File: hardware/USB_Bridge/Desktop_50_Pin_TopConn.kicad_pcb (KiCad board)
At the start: 2 copper layers, 89.2 x 82.6 mm, 108 parts, among them J1 Conn_01x03_Male, J10 Conn_01x03_Male, J11 ACK_En, J2 Conn_02x25_Odd_Even, J3 BergFloppy, J5 Conn_01x03_Male, J6 SM04B-SRSS-TB(LF)(SN), J7 TERM_BCKF, J8 EPWR, J9 Conn_01x02_Male, Q1 AO3401A, Q2 AO3401A, SW1 SW_MEC_5E, U13 LVT125, U14 LVT125, U15 LVT125, U16 LVT125, U3 AMS1117-2.85, U4 LVT245, U5 LVT245, U6 LVT245, U8 74HC14, U9 LVT245

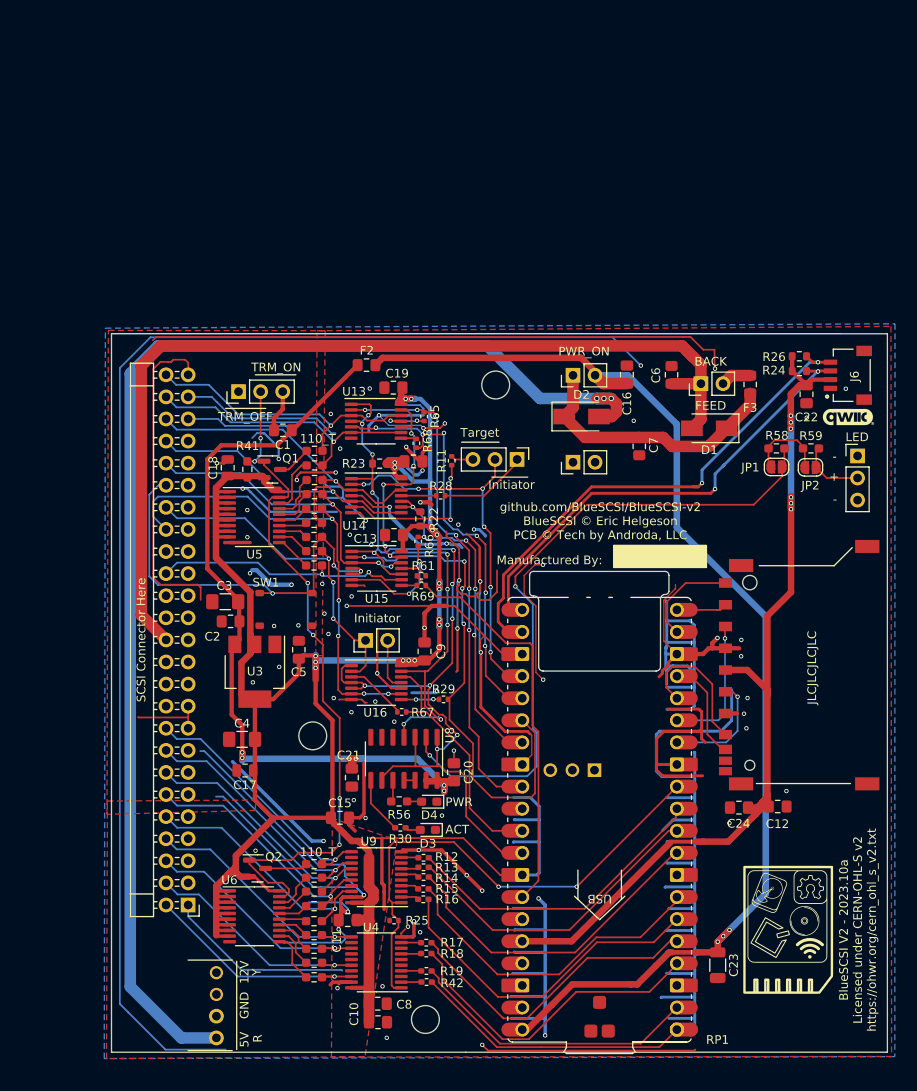
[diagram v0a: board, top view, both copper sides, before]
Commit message: intermediate checkin
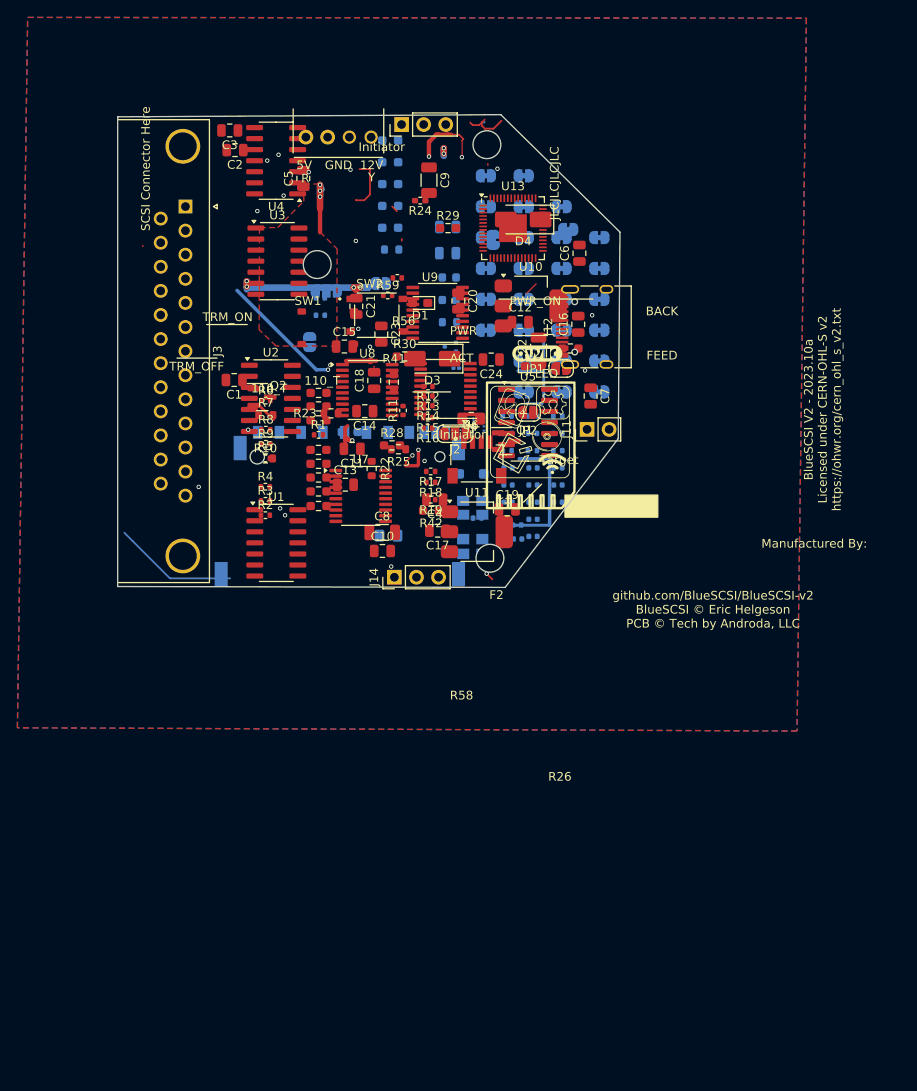
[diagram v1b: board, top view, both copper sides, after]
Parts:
- removed F3: Polyfuse, Fuse:Fuse_0805_2012Metric_Pad1.15x1.40mm_HandSolder
- removed J9: Conn_01x02_Male, Connector_PinHeader_2.54mm:PinHeader_1x02_P2.54mm_Vertical
- removed R61, R65, R66, R67, R68, R69: 1k, Resistor_SMD:R_0402_1005Metric
- removed RP1: PicoWModule, Library:Raspberry_Pi_PicoW_SMT_THT
- removed U14, U15, U16: LVT125, Package_SO:TSSOP-14_4.4x5mm_P0.65mm
- added C25: 10u 6.3V, Capacitor_SMD:C_0805_2012Metric, B.Cu at (138.6, 51.5)
- added C26: 10u 6.3V, Capacitor_SMD:C_0805_2012Metric, B.Cu at (138.6, 54.5)
- added C27: 2.2u 6.3V, Capacitor_SMD:C_0402_1005Metric, B.Cu at (151.3, 79.2)
- added C28: 100n 6.3V, Capacitor_SMD:C_0402_1005Metric, B.Cu at (151.3, 81.2)
- added C29: 100n 6.3V, Capacitor_SMD:C_0402_1005Metric, B.Cu at (151.3, 83.2)
- added C30: 100n 6.3V, Capacitor_SMD:C_0402_1005Metric, B.Cu at (144.9, 85.2)
- added C31: 2.2u 6.3V, Capacitor_SMD:C_0402_1005Metric, B.Cu at (142.1, 85.0)
- added C32: 2.2u 6.3V, Capacitor_SMD:C_0402_1005Metric, B.Cu at (146.6, 85.8)
- added C33: 100n 6.3V, Capacitor_SMD:C_0402_1005Metric, B.Cu at (148.5, 79.2)
- added C34: 100n 6.3V, Capacitor_SMD:C_0402_1005Metric, B.Cu at (148.5, 81.2)
- added C35: 100n 6.3V, Capacitor_SMD:C_0402_1005Metric, B.Cu at (148.5, 83.2)
- added C36: 100n 6.3V, Capacitor_SMD:C_0402_1005Metric, B.Cu at (148.5, 85.1)
- added C37: 100n 6.3V, Capacitor_SMD:C_0402_1005Metric, B.Cu at (148.5, 87.1)
- added C38: 2.2u 6.3V, Capacitor_SMD:C_0402_1005Metric, B.Cu at (146.7, 87.4)
- added C39: 100n 6.3V, Capacitor_SMD:C_0402_1005Metric, B.Cu at (145.6, 79.2)
- added C40: 100n 6.3V, Capacitor_SMD:C_0402_1005Metric, B.Cu at (145.6, 81.2)
- added C41: 1n 25V, Capacitor_SMD:C_0402_1005Metric, B.Cu at (145.6, 83.2)
- added D5: MBR120VLSFT1G, Diode_SMD:D_SOD-123F, B.Cu at (141.4, 79.9)
- added D6: Green, LED_SMD:LED_0603_1608Metric, B.Cu at (138.8, 57.3)
- added D7: Red, LED_SMD:LED_0603_1608Metric, B.Cu at (138.8, 59.9)
- added F1: Polyfuse, Fuse:Fuse_0805_2012Metric_Pad1.15x1.40mm_HandSolder, B.Cu at (131.8, 87.0)
- added J12: USB_C_Receptacle_USB2.0, Connector_USB:USB_C_Receptacle_HRO_TYPE-C-31-M-12, F.Cu at (155.9, 63.0)
- added J14: Debug, Connector_PinHeader_2.54mm:PinHeader_1x03_P2.54mm_Vertical, F.Cu at (132.5, 91.8)
- added J4: SM04B-SRSS-TB(LF)(SN), Library:JST_SM04B-SRSS-TB(LF)(SN), F.Cu at (142.0, 76.3)
- added JP16: SolderJumper_2_Bridged, Jumper:SolderJumper-2_P1.3mm_Bridged_RoundedPad1.0x1.5mm, B.Cu at (156.1, 52.7)
- added JP17: SolderJumper_2_Bridged, Jumper:SolderJumper-2_P1.3mm_Bridged_RoundedPad1.0x1.5mm, B.Cu at (156.1, 56.3)
- added JP18: SolderJumper_2_Bridged, Jumper:SolderJumper-2_P1.3mm_Bridged_RoundedPad1.0x1.5mm, B.Cu at (156.1, 59.8)
- added JP19: SolderJumper_2_Bridged, Jumper:SolderJumper-2_P1.3mm_Bridged_RoundedPad1.0x1.5mm, B.Cu at (156.1, 63.4)
- added JP20: SolderJumper_2_Bridged, Jumper:SolderJumper-2_P1.3mm_Bridged_RoundedPad1.0x1.5mm, B.Cu at (156.1, 66.9)
- added JP21: SolderJumper_2_Bridged, Jumper:SolderJumper-2_P1.3mm_Bridged_RoundedPad1.0x1.5mm, B.Cu at (156.1, 70.5)
- added JP24: SolderJumper_2_Bridged, Jumper:SolderJumper-2_P1.3mm_Bridged_RoundedPad1.0x1.5mm, B.Cu at (151.7, 49.2)
- added JP25: SolderJumper_2_Bridged, Jumper:SolderJumper-2_P1.3mm_Bridged_RoundedPad1.0x1.5mm, B.Cu at (151.7, 52.7)
- added JP26: SolderJumper_2_Bridged, Jumper:SolderJumper-2_P1.3mm_Bridged_RoundedPad1.0x1.5mm, B.Cu at (151.7, 56.3)
- added JP27: SolderJumper_2_Bridged, Jumper:SolderJumper-2_P1.3mm_Bridged_RoundedPad1.0x1.5mm, B.Cu at (151.7, 59.8)
- added JP28: SolderJumper_2_Bridged, Jumper:SolderJumper-2_P1.3mm_Bridged_RoundedPad1.0x1.5mm, B.Cu at (151.7, 63.4)
- added JP29: SolderJumper_2_Bridged, Jumper:SolderJumper-2_P1.3mm_Bridged_RoundedPad1.0x1.5mm, B.Cu at (151.7, 66.9)
- added JP3: SolderJumper_2_Bridged, Jumper:SolderJumper-2_P1.3mm_Bridged_RoundedPad1.0x1.5mm, B.Cu at (152.5, 51.8)
- added JP30: SolderJumper_2_Bridged, Jumper:SolderJumper-2_P1.3mm_Bridged_RoundedPad1.0x1.5mm, B.Cu at (151.7, 70.5)
- added JP32: SolderJumper_2_Bridged, Jumper:SolderJumper-2_P1.3mm_Bridged_RoundedPad1.0x1.5mm, B.Cu at (147.4, 45.6)
- added JP33: SolderJumper_2_Bridged, Jumper:SolderJumper-2_P1.3mm_Bridged_RoundedPad1.0x1.5mm, B.Cu at (147.4, 49.2)
- added JP34: SolderJumper_2_Bridged, Jumper:SolderJumper-2_P1.3mm_Bridged_RoundedPad1.0x1.5mm, B.Cu at (147.4, 52.7)
- added JP35: SolderJumper_2_Bridged, Jumper:SolderJumper-2_P1.3mm_Bridged_RoundedPad1.0x1.5mm, B.Cu at (147.4, 56.3)
- added JP36: SolderJumper_2_Bridged, Jumper:SolderJumper-2_P1.3mm_Bridged_RoundedPad1.0x1.5mm, B.Cu at (147.4, 59.8)
- added JP37: SolderJumper_2_Bridged, Jumper:SolderJumper-2_P1.3mm_Bridged_RoundedPad1.0x1.5mm, B.Cu at (147.4, 63.4)
- added JP38: SolderJumper_2_Bridged, Jumper:SolderJumper-2_P1.3mm_Bridged_RoundedPad1.0x1.5mm, B.Cu at (147.4, 66.9)
- added JP39: SolderJumper_2_Bridged, Jumper:SolderJumper-2_P1.3mm_Bridged_RoundedPad1.0x1.5mm, B.Cu at (147.4, 70.5)
- added JP40: SolderJumper_2_Bridged, Jumper:SolderJumper-2_P1.3mm_Bridged_RoundedPad1.0x1.5mm, B.Cu at (143.0, 42.1)
- added JP41: SolderJumper_2_Bridged, Jumper:SolderJumper-2_P1.3mm_Bridged_RoundedPad1.0x1.5mm, B.Cu at (143.0, 45.6)
- added JP42: SolderJumper_2_Bridged, Jumper:SolderJumper-2_P1.3mm_Bridged_RoundedPad1.0x1.5mm, B.Cu at (143.0, 49.2)
- added JP43: SolderJumper_2_Bridged, Jumper:SolderJumper-2_P1.3mm_Bridged_RoundedPad1.0x1.5mm, B.Cu at (143.0, 52.7)
- added JP44: SolderJumper_2_Bridged, Jumper:SolderJumper-2_P1.3mm_Bridged_RoundedPad1.0x1.5mm, B.Cu at (143.0, 56.3)
- added JP45: SolderJumper_2_Bridged, Jumper:SolderJumper-2_P1.3mm_Bridged_RoundedPad1.0x1.5mm, B.Cu at (143.0, 59.8)
- added JP46: SolderJumper_2_Bridged, Jumper:SolderJumper-2_P1.3mm_Bridged_RoundedPad1.0x1.5mm, B.Cu at (143.0, 63.4)
- added Q3: DMG1012T, Package_TO_SOT_SMD:SOT-523, B.Cu at (139.0, 65.3)
- added R20: 1k, Resistor_SMD:R_0402_1005Metric, B.Cu at (124.0, 59.7)
- added R21: 1k, Resistor_SMD:R_0402_1005Metric, B.Cu at (124.0, 61.7)
- added R27: 330, Resistor_SMD:R_0603_1608Metric_Pad0.98x0.95mm_HandSolder, B.Cu at (127.4, 75.1)
- added R31: 110, Resistor_SMD:R_0603_1608Metric_Pad0.98x0.95mm_HandSolder, B.Cu at (132.0, 41.6)
- added R32: 110, Resistor_SMD:R_0603_1608Metric_Pad0.98x0.95mm_HandSolder, B.Cu at (132.0, 44.1)
- added R43: 110, Resistor_SMD:R_0603_1608Metric_Pad0.98x0.95mm_HandSolder, B.Cu at (132.0, 46.6)
- added R44: 110, Resistor_SMD:R_0603_1608Metric_Pad0.98x0.95mm_HandSolder, B.Cu at (132.0, 49.1)
- added R45: 110, Resistor_SMD:R_0603_1608Metric_Pad0.98x0.95mm_HandSolder, B.Cu at (132.0, 51.6)
- added R46: 4.7k, Resistor_SMD:R_0603_1608Metric, B.Cu at (132.2, 54.1)
- added R47: 5.1k, Resistor_SMD:R_0402_1005Metric, B.Cu at (151.3, 73.3)
- added R48: 5.1k, Resistor_SMD:R_0402_1005Metric, B.Cu at (151.3, 75.3)
- added R49: 5.6k, Resistor_SMD:R_0402_1005Metric, B.Cu at (151.3, 77.2)
- added R50: 200R, Resistor_SMD:R_0603_1608Metric, B.Cu at (138.9, 62.5)
- added R51: 10k, Resistor_SMD:R_0402_1005Metric, B.Cu at (148.4, 73.3)
- added R52: 1R, Resistor_SMD:R_0402_1005Metric, B.Cu at (148.4, 75.3)
- added R53: 470R, Resistor_SMD:R_0402_1005Metric, B.Cu at (148.4, 77.2)
- added R54: 470R, Resistor_SMD:R_0402_1005Metric, B.Cu at (145.5, 73.3)
- added R55: NO-FIT, Resistor_SMD:R_0402_1005Metric, B.Cu at (145.5, 75.3)
- added R57: 27R, Resistor_SMD:R_0201_0603Metric, B.Cu at (139.6, 67.8)
- added R60: 100k, Resistor_SMD:R_0402_1005Metric, B.Cu at (145.5, 77.2)
- added SW2: TS-1187A-B-A-B, TS-1187A-B-A-B:SW_TS-1187A-B-A-B, F.Cu at (130.5, 61.7)
- added U1: LVT125, Package_SO:SO-14_3.9x8.65mm_P1.27mm, F.Cu at (119.0, 87.8)
- added U10: AMS1117-2.85, Package_TO_SOT_SMD:SOT-223-3_TabPin2, F.Cu at (148.2, 60.6)
- added U11: AMS1117-3.3, Package_TO_SOT_SMD:SOT-223-3_TabPin2, F.Cu at (142.0, 86.6)
- added U12: W25Q16JVUXIQ, agausmann:USON-8-1EP_3x2mm_P0.5mm_EP0.2x1.6mm, B.Cu at (141.6, 74.2)
- added U2: LVT125, Package_SO:SO-14_3.9x8.65mm_P1.27mm, F.Cu at (118.3, 71.2)
- added U7: LVT245, Package_SO:TSSOP-20_4.4x6.5mm_P0.65mm, F.Cu at (128.7, 82.5)
- added X1: SIT1602AI-22-33E-12.000000, Crystal:Crystal_SMD_SeikoEpson_TSX3225-4Pin_3.2x2.5mm, B.Cu at (141.5, 83.8)
- added Y1: 12MHz, Crystal:Crystal_SMD_3225-4Pin_3.2x2.5mm, B.Cu at (141.5, 88.3)
- C1, C2, C5, C7: footprint Capacitor_SMD:C_0805_2012Metric_Pad1.15x1.40mm_HandSolder -> Capacitor_SMD:C_0805_2012Metric
- C10, C15, C16: value 4.7uF -> 0.1uF; footprint Capacitor_SMD:C_0805_2012Metric_Pad1.18x1.45mm_HandSolder -> Capacitor_SMD:C_0805_2012Metric
- C11, C13, C14, C21: footprint Capacitor_SMD:C_0805_2012Metric_Pad1.18x1.45mm_HandSolder -> Capacitor_SMD:C_0805_2012Metric
- C12, C6: value 4.7uF -> 0.1uF; footprint Capacitor_SMD:C_0805_2012Metric_Pad1.15x1.40mm_HandSolder -> Capacitor_SMD:C_0805_2012Metric
- C17: value 0.1uF -> 4.7uF
- C19, C20, C24: value 0.1uF -> 4.7uF; footprint Capacitor_SMD:C_0805_2012Metric_Pad1.18x1.45mm_HandSolder -> Capacitor_SMD:C_0805_2012Metric
- C22, C8, C9: value 0.1uF -> 20uF; footprint Capacitor_SMD:C_0805_2012Metric_Pad1.18x1.45mm_HandSolder -> Capacitor_SMD:C_1206_3216Metric
- C23: value 20uF -> 0.1uF; footprint Capacitor_SMD:C_1206_3216Metric -> Capacitor_SMD:C_0805_2012Metric
- C3: value 20uF -> 4.7uF; footprint Capacitor_SMD:C_1206_3216Metric_Pad1.42x1.75mm_HandSolder -> Capacitor_SMD:C_0805_2012Metric
- C4: value 20uF -> 0.1uF; footprint Capacitor_SMD:C_1206_3216Metric_Pad1.42x1.75mm_HandSolder -> Capacitor_SMD:C_0805_2012Metric
- D1, D2: value D -> LED; footprint Diode_SMD:D_SMA -> LED_SMD:LED_0603_1608Metric_Pad1.05x0.95mm_HandSolder
- D3, D4: value LED -> D; footprint LED_SMD:LED_0603_1608Metric_Pad1.05x0.95mm_HandSolder -> Diode_SMD:D_SMA
- J1: value Conn_01x03_Male -> ACK_En; footprint Connector_PinHeader_2.54mm:PinHeader_1x03_P2.54mm_Vertical -> Jumper:SolderJumper-2_P1.3mm_Open_RoundedPad1.0x1.5mm; moved to B.Cu
- J10: value Conn_01x03_Male -> BergFloppy; footprint Connector_PinHeader_2.54mm:PinHeader_1x03_P2.54mm_Vertical -> Library:BergFloppy_RightAngle
- J11: value ACK_En -> Conn_01x02_Male
- J2: value Conn_02x25_Odd_Even -> Conn_01x03_Male; footprint Connector_PinHeader_2.54mm:PinHeader_2x25_P2.54mm_Horizontal -> Jumper:SolderJumper-3_P1.3mm_Open_RoundedPad1.0x1.5mm
- J3: value BergFloppy -> DB25_Plug_MountingHoles; footprint CustomFootprints:BergFloppy_RightAngle -> Connector_Dsub:DSUB-25_Male_Horizontal_P2.77x2.84mm_EdgePinOffset4.94mm_Housed_MountingHolesOffset7.48mm
- J6: value SM04B-SRSS-TB(LF)(SN) -> Conn_01x03_Male; footprint Library:JST_SM04B-SRSS-TB(LF)(SN) -> Jumper:SolderJumper-3_P1.3mm_Open_RoundedPad1.0x1.5mm; moved to B.Cu
- J7, J8: footprint Connector_PinHeader_2.54mm:PinHeader_1x02_P2.54mm_Vertical -> Jumper:SolderJumper-2_P1.3mm_Open_RoundedPad1.0x1.5mm; moved to B.Cu
- R1, R10, R2, R3, R4, R6, R8, R9: value 110 -> 1k; footprint Resistor_SMD:R_0603_1608Metric_Pad0.98x0.95mm_HandSolder -> Resistor_SMD:R_0402_1005Metric
- R12, R13, R14, R15, R16, R17, R18, R19: footprint Resistor_SMD:R_0402_1005Metric_Pad0.72x0.64mm_HandSolder -> Resistor_SMD:R_0402_1005Metric
- R24: value 4.7k -> 470; footprint Resistor_SMD:R_0603_1608Metric -> Resistor_SMD:R_0402_1005Metric_Pad0.72x0.64mm_HandSolder
- R25: value 1k -> 4.7k; footprint Resistor_SMD:R_0402_1005Metric -> Resistor_SMD:R_0603_1608Metric
- R26: value 4.7k -> 150; footprint Resistor_SMD:R_0603_1608Metric -> Resistor_SMD:R_0603_1608Metric_Pad0.98x0.95mm_HandSolder
- R28, R29: value 1k -> 110; footprint Resistor_SMD:R_0402_1005Metric -> Resistor_SMD:R_0603_1608Metric_Pad0.98x0.95mm_HandSolder
- R30: value 470 -> 110; footprint Resistor_SMD:R_0402_1005Metric_Pad0.72x0.64mm_HandSolder -> Resistor_SMD:R_0603_1608Metric_Pad0.98x0.95mm_HandSolder
- R41: value 4.7k -> 110
- R42: value 1k -> 110; footprint Resistor_SMD:R_0402_1005Metric_Pad0.72x0.64mm_HandSolder -> Resistor_SMD:R_0603_1608Metric_Pad0.98x0.95mm_HandSolder
- R5, R7: value 110 -> 4.7k; footprint Resistor_SMD:R_0603_1608Metric_Pad0.98x0.95mm_HandSolder -> Resistor_SMD:R_0603_1608Metric
- R56: value 4.7k -> 27R; footprint Resistor_SMD:R_0603_1608Metric_Pad0.98x0.95mm_HandSolder -> Resistor_SMD:R_0201_0603Metric
- R58: value 150 -> 1k; footprint Resistor_SMD:R_0603_1608Metric_Pad0.98x0.95mm_HandSolder -> Resistor_SMD:R_0402_1005Metric
- R59: value 330 -> 200k; footprint Resistor_SMD:R_0603_1608Metric_Pad0.98x0.95mm_HandSolder -> Resistor_SMD:R_0402_1005Metric
- SD1: moved to B.Cu
- U13: value LVT125 -> RP2040; footprint Package_SO:TSSOP-14_4.4x5mm_P0.65mm -> Package_DFN_QFN:QFN-56-1EP_7x7mm_P0.4mm_EP3.2x3.2mm
- U3: value AMS1117-2.85 -> LVT125; footprint Package_TO_SOT_SMD:SOT-223-3_TabPin2 -> Package_SO:SO-14_3.9x8.65mm_P1.27mm
- U4: value LVT245 -> LVT125; footprint Package_SO:TSSOP-20_4.4x6.5mm_P0.65mm -> Package_SO:SO-14_3.9x8.65mm_P1.27mm
- U5: value LVT245 -> 74HC14; footprint Package_SO:TSSOP-20_4.4x6.5mm_P0.65mm -> Package_SO:SOIC-14_3.9x8.7mm_P1.27mm
- U8: value 74HC14 -> LVT245; footprint Package_SO:SO-14_3.9x8.65mm_P1.27mm -> Package_SO:TSSOP-20_4.4x6.5mm_P0.65mm
- moved U4 92.9 mm to (118.9, 43.9)
- moved J3 92.2 mm to (108.5, 49.2)
- moved C23 82.2 mm to (131.0, 63.9)
- moved D4 67.8 mm to (147.3, 50.7)
- moved U9 65.3 mm to (137.5, 61.4)
- moved J5 64.8 mm to (133.3, 39.8), turned to 90 degrees
- moved U6 64.5 mm to (138.4, 70.2), turned to 180 degrees
- moved C12 63.1 mm to (147.0, 62.5)
- moved G*** 63.1 mm to (148.2, 76.6)
- moved J2 62.3 mm to (139.5, 75.3)
- moved C24 58.9 mm to (143.7, 66.8)
- moved J6 58.8 mm to (124.7, 58.9), turned to 0 degrees
- moved R18 54.2 mm to (136.7, 80.9)
- moved R38 54.2 mm to (123.8, 80.3)
- moved R42 54.2 mm to (136.7, 84.2)
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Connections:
- C1 pad 1: +5F -> GND
- C1 pad 2: GND -> +3V3
- C11 pad 1: +2V8 -> +5F
- C12 pad 1: +3V3 -> +5F
- C15 pad 1: +2V8 -> GND
- C15 pad 2: GND -> +2V8
- C16 pad 1: +5VP -> GND
- C16 pad 2: GND -> +2V8
- C17 pad 1: +2V8 -> +3V3
- C18 pad 1: +2V8 -> +3V3
- C19 pad 1: GND -> +5V
- C19 pad 2: +2V8 -> GND
- C2 pad 1: +5F -> +2V8
- C20 pad 1: GND -> Net-(D3-K)
- C20 pad 2: +5F -> GND
- C21 pad 1: +5F -> +5VP
- C22 pad 1: GND -> +5VP
- C22 pad 2: +3V3 -> GND
- C23 pad 1: +5VP -> GND
- C23 pad 2: GND -> +5F
- C24 pad 1: +3V3 -> +5F
- C3 pad 1: +5F -> +2V8
- C6 pad 1: +5V -> +2V8
- C7 pad 1: Net-(C7-Pad1) -> +2V8
- C8 pad 1: +2V8 -> +5F
- C9 pad 1: GND -> +2V8
- C9 pad 2: +2V8 -> GND
- D1 pad 1: Net-(C7-Pad1) -> GND
- D1 pad 2: +5V -> Net-(D1-A)
- D2 pad 1: Net-(C7-Pad1) -> GND
- D2 pad 2: Net-(D2-Pad2) -> Net-(D2-A)
- D3 pad 1: GND -> Net-(D3-K)
- D3 pad 2: Net-(D3-Pad2) -> +5V
- D4 pad 1: GND -> Net-(D3-K)
- D4 pad 2: Net-(D4-Pad2) -> Net-(D4-A)
- J1 pad 1: unconnected-(J1-Pad1) -> ACK
- J1 pad 2: TRM_ON_J -> ACKDr
- J10 pad 1: Net-(J10-Pad1) -> Net-(D4-A)
- J10 pad 2: oCD_iSEL -> GND
- J10 pad 3: Net-(J10-Pad3) -> GND
- J11 pad 1: ACK -> GND
- J11 pad 2: ACKDr -> GND
- J2 pad 1: GND -> Net-(J2-Pin_1)
- J2 pad 2: DB0 -> oCD_iSEL
- J2 pad 3: GND -> Net-(J2-Pin_3)
- J3 pad 1: Net-(D2-Pad2) -> REQ
- J3 pad 2: GND -> MSG
- J3 pad 3: GND -> IO
- J3 pad 4: unconnected-(J3-Pad4) -> RST
- J5 pad 2: Net-(J5-Pad2) -> Net-(J5-Pin_2)
- J6 pad 1: GND -> unconnected-(J6-Pin_1-Pad1)
- J6 pad 2: +3V3 -> TRM_ON_J
- J6 pad 3: SDA -> GND
- J8 pad 1: Net-(C7-Pad1) -> Net-(D3-K)
- JP1 pad 1: Net-(JP1-Pad1) -> Net-(JP1-A)
- JP1 pad 2: Net-(JP1-Pad2) -> Net-(J5-Pin_2)
- JP2 pad 1: Net-(JP1-Pad2) -> Net-(JP2-A)
- JP2 pad 2: Net-(J5-Pad2) -> Net-(JP1-A)
- Q1 pad 3: Net-(Q1-Pad3) -> Net-(Q1-D)
- Q2 pad 3: Net-(Q2-Pad3) -> Net-(Q2-D)
- R1 pad 1: Net-(R1-Pad1) -> iSEL
- R1 pad 2: DB5 -> Net-(J2-Pin_3)
- R10 pad 1: Net-(R10-Pad1) -> Net-(RP1-G8)
- R10 pad 2: BSY -> DBPT
- R11 pad 1: iSEL -> oACK
- R11 pad 2: Net-(J10-Pad3) -> iACK
- R12 pad 2: DBPT -> DB7T
- R13 pad 2: DB7T -> DB6T
- R14 pad 2: DB6T -> DB5T
- R15 pad 1: Net-(R15-Pad1) -> Net-(RP1-G28)
- R15 pad 2: DB5T -> iATN
- R19 pad 1: Net-(R19-Pad1) -> Net-(RP1-G28)
- R19 pad 2: DB1T -> iMSG
- R2 pad 1: Net-(R2-Pad1) -> iCD
- R2 pad 2: ATN -> Net-(J2-Pin_1)
- R22 pad 1: oSEL -> SDA
- R22 pad 2: +2V8 -> +3V3
- R23 pad 1: oBSY -> +3V3
- R23 pad 2: +2V8 -> SCL
- R24 pad 1: SDA -> Net-(R24-Pad1)
- R24 pad 2: +3V3 -> Net-(D1-A)
- R25 pad 1: DBPTr -> Net-(R25-Pad1)
- R25 pad 2: GND -> Net-(D2-A)
- R26 pad 1: +3V3 -> Net-(JP2-A)
- R26 pad 2: SCL -> Net-(JP1-A)
- R28 pad 1: iCD -> Net-(U7-B1)
- R28 pad 2: Net-(J10-Pad1) -> REQ
- R29 pad 1: iBSY -> Net-(U8-B1)
- R29 pad 2: oMSG_iBSY -> DB7
- R3 pad 1: Net-(R3-Pad1) -> oREQ
- R3 pad 2: ACK -> iREQ
- R30 pad 1: Net-(R30-Pad1) -> Net-(U7-B2)
- R30 pad 2: Net-(D3-Pad2) -> CD
- R33 pad 1: Net-(R33-Pad1) -> Net-(U8-B3)
- R33 pad 2: DB6 -> DB5
- R34 pad 1: Net-(R34-Pad1) -> Net-(U7-B4)
- R34 pad 2: DB7 -> BSY
- R35 pad 1: Net-(Q2-Pad3) -> Net-(U8-B4)
- R35 pad 2: DBP -> DB4
- R36 pad 1: Net-(R36-Pad1) -> Net-(U7-B5)
- R36 pad 2: DB0 -> SEL
- R37 pad 1: Net-(R37-Pad1) -> Net-(U8-B5)
- R37 pad 2: DB1 -> DB3
- R38 pad 1: Net-(R38-Pad1) -> Net-(U7-B6)
- R38 pad 2: DB2 -> RST
- R39 pad 1: Net-(R39-Pad1) -> Net-(U8-B6)
- R39 pad 2: DB3 -> DB2
- R4 pad 1: Net-(R4-Pad1) -> iBSY
- R4 pad 2: RST -> oMSG_iBSY
- R40 pad 1: Net-(R40-Pad1) -> Net-(U7-B7)
- R40 pad 2: DB4 -> ACK
- R41 pad 1: TRM_ON_J -> Net-(U8-B7)
- R41 pad 2: +2V8 -> DB1
- R42 pad 2: DB0T -> ATN
- R5 pad 1: Net-(R5-Pad1) -> oSEL
- R5 pad 2: SEL -> +2V8
- R56 pad 1: Net-(R56-Pad1) -> /piccolo/USB_D+
- R56 pad 2: Net-(D4-Pad2) -> Net-(JP18-A)
- R58 pad 1: Net-(JP1-Pad1) -> /piccolo/QSPI_SS
- R58 pad 2: Net-(JP1-Pad2) -> Net-(R58-Pad2)
- R59 pad 1: Net-(JP1-Pad2) -> /piccolo/VSYS
- R59 pad 2: Net-(J5-Pad2) -> Net-(Q3-D)
- R6 pad 1: Net-(Q1-Pad3) -> iRST
- R6 pad 2: IO -> oSEL
- R7 pad 1: Net-(R7-Pad1) -> oBSY
- R7 pad 2: REQ -> +2V8
- R8 pad 1: Net-(R8-Pad1) -> iIO
- R8 pad 2: CD -> oIO
- R9 pad 1: Net-(R9-Pad1) -> DBPTr
- R9 pad 2: MSG -> GND
- U13 pad 1: oBSY -> +3V3
- U13 pad 10: !oBSY -> +3V3
- U13 pad 11: iIO -> Net-(JP19-A)
- U13 pad 12: IO -> Net-(JP21-A)
- U13 pad 13: !oBSY -> Net-(JP23-A)
- U13 pad 14: +2V8 -> Net-(JP24-A)
- U13 pad 2: oIO -> Net-(JP4-A)
- U13 pad 3: IO -> Net-(JP6-A)
- U13 pad 4: oBSY -> Net-(JP8-A)
- U13 pad 5: oREQ -> Net-(JP10-A)
- U13 pad 6: REQ -> Net-(JP12-A)
- U13 pad 7: GND -> Net-(JP14-A)
- U13 pad 8: iREQ -> Net-(JP15-A)
- U13 pad 9: REQ -> Net-(JP17-A)
- U3 pad 1: GND -> oBSY
- U3 pad 2: +2V8 -> oMSG_iBSY
- U3 pad 3: +5F -> MSG
- U4 pad 1: DBPTr -> oBSY
- U4 pad 11: DB3 -> ACKDr
- U4 pad 12: unconnected-(U4-Pad12) -> oACK
- U4 pad 13: DB2 -> !oBSY
- U4 pad 14: unconnected-(U4-Pad14) -> +2V8
- U4 pad 2: DB0T -> ACK
- U4 pad 3: unconnected-(U4-Pad3) -> iACK
- U4 pad 4: DB1T -> oBSY
- U4 pad 5: unconnected-(U4-Pad5) -> oBSY
- U4 pad 6: unconnected-(U4-Pad6) -> BSY
- U4 pad 7: DB2T -> GND
- U4 pad 8: unconnected-(U4-Pad8) -> iBSY
- U4 pad 9: DB3T -> BSY
- U5 pad 1: +2V8 -> oBSY
- U5 pad 10: GND -> Net-(R25-Pad1)
- U5 pad 11: Net-(R2-Pad1) -> Net-(U5-Pad11)
- U5 pad 12: Net-(R3-Pad1) -> Net-(U5-Pad11)
- U5 pad 13: Net-(R4-Pad1) -> +5F
- U5 pad 14: Net-(R5-Pad1) -> +5F
- U5 pad 2: +2V8 -> Net-(JP2-A)
- U5 pad 3: +2V8 -> oBSY
- U5 pad 4: +2V8 -> !oBSY
- U5 pad 5: +2V8 -> GND
- U5 pad 6: +2V8 -> unconnected-(U5-Pad6)
- U5 pad 7: +2V8 -> GND
- U5 pad 8: +2V8 -> Net-(R24-Pad1)
- U5 pad 9: +2V8 -> oBSY
- U6 pad 1: +2V8 -> DBPTr
- U6 pad 11: Net-(R36-Pad1) -> DB3
- U6 pad 12: Net-(R37-Pad1) -> unconnected-(U6-B7-Pad12)
- U6 pad 13: Net-(R38-Pad1) -> DB2
- U6 pad 14: Net-(R39-Pad1) -> unconnected-(U6-B5-Pad14)
- U6 pad 15: Net-(R40-Pad1) -> unconnected-(U6-B4-Pad15)
- U6 pad 16: Net-(R1-Pad1) -> DB1
- U6 pad 17: Net-(R33-Pad1) -> unconnected-(U6-B2-Pad17)
- U6 pad 18: Net-(R34-Pad1) -> DB0
- U6 pad 19: TRM_ON_J -> GND
- U6 pad 2: +2V8 -> DB0T
- U6 pad 3: +2V8 -> unconnected-(U6-A2-Pad3)
- U6 pad 4: +2V8 -> DB1T
- U6 pad 5: +2V8 -> unconnected-(U6-A4-Pad5)
- U6 pad 6: +2V8 -> unconnected-(U6-A5-Pad6)
- U6 pad 7: +2V8 -> DB2T
- U6 pad 8: +2V8 -> unconnected-(U6-A7-Pad8)
- U6 pad 9: +2V8 -> DB3T
- U8 pad 1: oBSY -> +2V8
- U8 pad 10: Net-(R56-Pad1) -> GND
- U8 pad 11: Net-(U8-Pad11) -> Net-(U8-B8)
- U8 pad 12: Net-(U8-Pad11) -> Net-(U8-B7)
- U8 pad 13: +5F -> Net-(U8-B6)
- U8 pad 14: +5F -> Net-(U8-B5)
- U8 pad 2: Net-(JP1-Pad1) -> +2V8
- U8 pad 3: oBSY -> +2V8
- U8 pad 4: !oBSY -> +2V8
- U8 pad 5: GND -> +2V8
- U8 pad 6: unconnected-(U8-Pad6) -> +2V8
- U8 pad 7: GND -> +2V8
- U8 pad 8: Net-(R30-Pad1) -> +2V8
- U8 pad 9: oBSY -> +2V8
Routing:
- net GND: track 948.6 -> 92.2 mm, vias 81 -> 26
- net +2V8: track 259.3 -> 21.6 mm, vias 16 -> 5
- net Net-(D2-Pad2): track 151.4 -> 0.00 mm, vias 3 -> 0
- net +5VP: track 144.9 -> 0.00 mm, vias 3 -> 0
- net oBSY: track 114.8 -> 0.00 mm, vias 12 -> 0
- net +5V: track 112.6 -> 0.00 mm
- net +3V3: track 109.8 -> 0.00 mm, vias 6 -> 0
- net +5F: track 93.3 -> 0.00 mm, vias 6 -> 0
- net TRM_ON_J: track 79.9 -> 0.00 mm, vias 6 -> 0
- net Net-(JP1-Pad1): track 77.8 -> 0.00 mm, vias 2 -> 0
- net !oBSY: track 61.1 -> 0.00 mm, vias 10 -> 0
- net oIO: track 59.3 -> 0.00 mm, vias 6 -> 0
- net DBPTr: track 59.2 -> 0.00 mm, vias 2 -> 0
- net SCL: track 58.1 -> 0.00 mm, vias 2 -> 0
- net oMSG_iBSY: track 58.0 -> 0.00 mm, vias 4 -> 0
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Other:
- board size 89.2 x 82.6 mm -> 57.8 x 54.4 mm
